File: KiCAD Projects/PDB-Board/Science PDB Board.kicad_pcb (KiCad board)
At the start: 2 copper layers, 85.1 x 63.5 mm, 8 parts, among them P1 MOTOR_PWR_OUT, P2 MAIN_PWR_IN, P3 5V_OUT, P4 PWR_REG

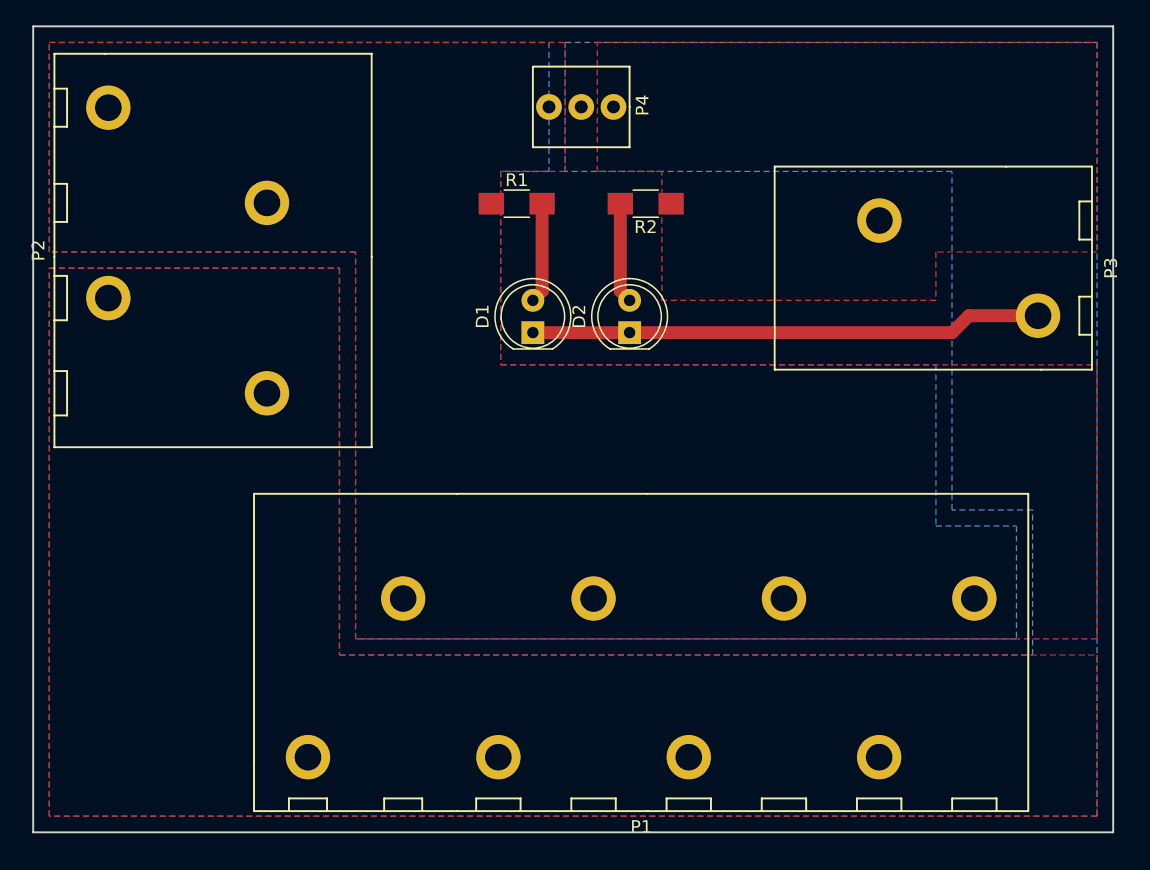
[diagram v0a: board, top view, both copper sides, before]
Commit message: Finished? PDB v2
Committing this that weren't?
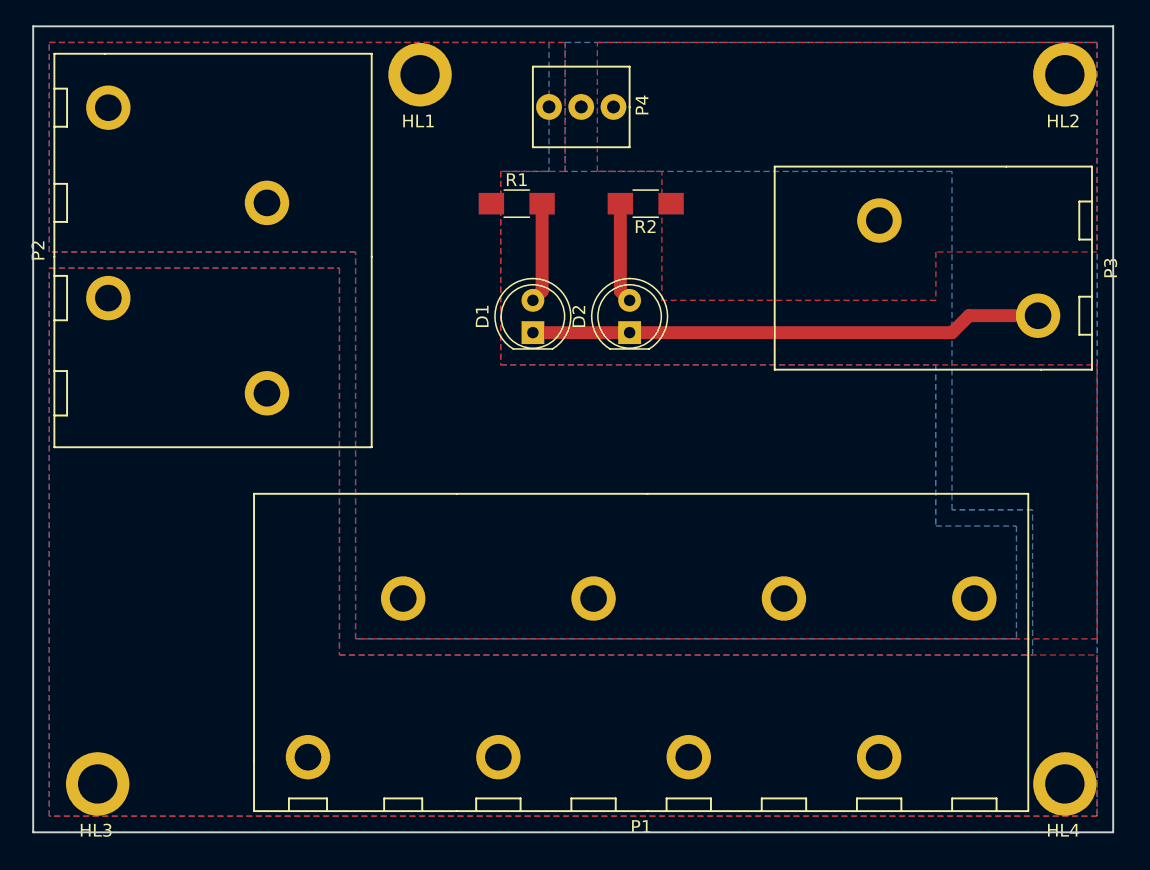
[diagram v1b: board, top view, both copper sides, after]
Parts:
- added HL1: HOLE, hole:HOLE_M3, F.Cu at (144.8, 80.0)
- added HL2: HOLE, hole:HOLE_M3, F.Cu at (195.6, 80.0)
- added HL3: HOLE, hole:HOLE_M3, F.Cu at (119.4, 135.9)
- added HL4: HOLE, hole:HOLE_M3, F.Cu at (195.6, 135.9)
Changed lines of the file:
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@@
 (kicad_pcb (version 4) (host pcbnew 4.0.3-stable)
   (general
-    (links 20)
-    (no_connects 0)
+    (links 24)
+    (no_connects 1)
     (area 114.224999 76.124999 199.465001 139.775001)
     (thickness 1.6)
@@
     (tracks 8)
     (zones 0)
-    (modules 8)
+    (modules 12)
     (nets 6)
   )
@@
   )
   (setup
-    (last_trace_width 1.016)
+    (last_trace_width 0.25)
     (user_trace_width 1.016)
     (trace_clearance 0.2)
@@
     )
   )
+  (module hole:HOLE_M3 (layer F.Cu)
+    (at 144.78 80.01)
+    (fp_text reference HL1 (at -0.127 3.683) (layer F.SilkS)
+      (effects (font (size 1 1) (thickness 0.15)))
+    )
+    (fp_text value HOLE (at 0.127 -3.683) (layer F.Fab)
+      (effects (font (size 1 1) (thickness 0.15)))
+    )
+    (pad 1 thru_hole circle (at 0 0) (size 5 5) (drill 3.1) (layers *.Cu *.Mask)
+      (net 5 GND))
+  )
+  (module hole:HOLE_M3 (layer F.Cu)
+    (at 195.58 80.01)
+    (fp_text reference HL2 (at -0.127 3.683) (layer F.SilkS)
+      (effects (font (size 1 1) (thickness 0.15)))
+    )
+    (fp_text value HOLE (at 0.127 -3.683) (layer F.Fab)
+      (effects (font (size 1 1) (thickness 0.15)))
+    )
+    (pad 1 thru_hole circle (at 0 0) (size 5 5) (drill 3.1) (layers *.Cu *.Mask)
+      (net 5 GND))
+  )
+  (module hole:HOLE_M3 (layer F.Cu)
+    (at 119.38 135.89)
+    (fp_text reference HL3 (at -0.127 3.683) (layer F.SilkS)
+      (effects (font (size 1 1) (thickness 0.15)))
+    )
+    (fp_text value HOLE (at 0.127 -3.683) (layer F.Fab)
+      (effects (font (size 1 1) (thickness 0.15)))
+    )
+    (pad 1 thru_hole circle (at 0 0) (size 5 5) (drill 3.1) (layers *.Cu *.Mask)
+      (net 5 GND))
+  )
+  (module hole:HOLE_M3 (layer F.Cu)
+    (at 195.58 135.89)
+    (fp_text reference HL4 (at -0.127 3.683) (layer F.SilkS)
+      (effects (font (size 1 1) (thickness 0.15)))
+    )
+    (fp_text value HOLE (at 0.127 -3.683) (layer F.Fab)
+      (effects (font (size 1 1) (thickness 0.15)))
+    )
+    (pad 1 thru_hole circle (at 0 0) (size 5 5) (drill 3.1) (layers *.Cu *.Mask)
+      (net 5 GND))
+  )
   (gr_line (start 114.3 139.7) (end 114.3 76.2) (angle 90) (layer Edge.Cuts) (width 0.15))
   (gr_line (start 199.39 139.7) (end 114.3 139.7) (angle 90) (layer Edge.Cuts) (width 0.15))
@@
   (segment (start 160.56 90.17) (end 160.56 97.06) (width 1.016) (layer F.Cu) (net 4))
   (segment (start 160.56 97.06) (end 161.29 97.79) (width 1.016) (layer F.Cu) (net 4))
-  (segment (start 153.67 100.33) (end 161.29 100.33) (width 1.016) (layer F.Cu) (net 5) (status C00000))
-  (segment (start 161.29 100.33) (end 186.69 100.33) (width 1.016) (layer F.Cu) (net 5) (status 400000))
+  (segment (start 153.67 100.33) (end 161.29 100.33) (width 1.016) (layer F.Cu) (net 5))
+  (segment (start 161.29 100.33) (end 186.69 100.33) (width 1.016) (layer F.Cu) (net 5))
   (segment (start 186.69 100.33) (end 188.02 99) (width 1.016) (layer F.Cu) (net 5))
-  (segment (start 188.02 99) (end 193.47 99) (width 1.016) (layer F.Cu) (net 5) (status 800000))
+  (segment (start 188.02 99) (end 193.47 99) (width 1.016) (layer F.Cu) (net 5))
   (zone (net 3) (net_name +5V) (layer F.Cu) (hatch edge 0.508)
     (connect_pads (clearance 0.508))

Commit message: Revert "Finished? PDB v2"
This reverts commit a04adeda8b22dfbdd33fba7944ab085dcccc9394.
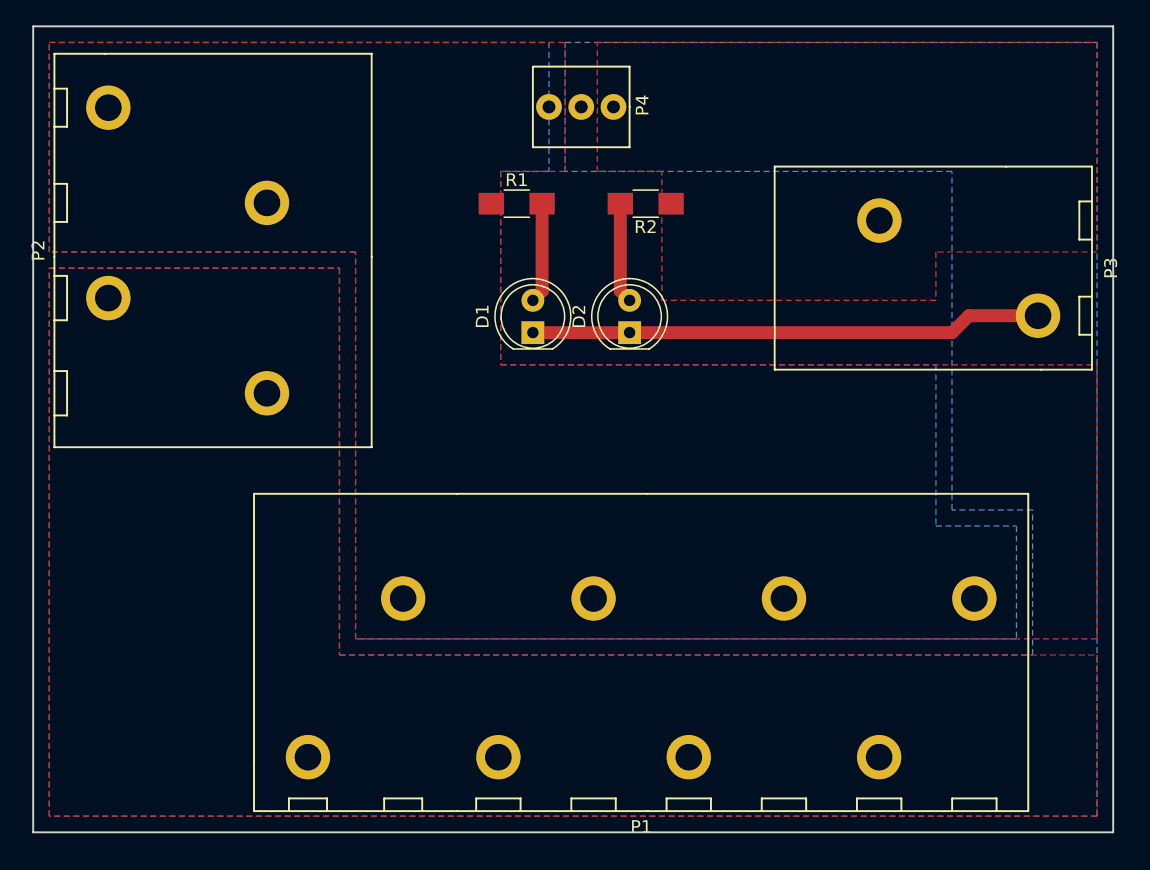
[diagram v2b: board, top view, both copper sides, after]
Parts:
- removed HL1, HL2, HL3, HL4: HOLE, hole:HOLE_M3
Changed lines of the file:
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@@
 (kicad_pcb (version 4) (host pcbnew 4.0.3-stable)
   (general
-    (links 24)
-    (no_connects 1)
+    (links 20)
+    (no_connects 0)
     (area 114.224999 76.124999 199.465001 139.775001)
     (thickness 1.6)
@@
     (tracks 8)
     (zones 0)
-    (modules 12)
+    (modules 8)
     (nets 6)
   )
@@
   )
   (setup
-    (last_trace_width 0.25)
+    (last_trace_width 1.016)
     (user_trace_width 1.016)
     (trace_clearance 0.2)
@@
     )
   )
-  (module hole:HOLE_M3 (layer F.Cu)
-    (at 144.78 80.01)
-    (fp_text reference HL1 (at -0.127 3.683) (layer F.SilkS)
-      (effects (font (size 1 1) (thickness 0.15)))
-    )
-    (fp_text value HOLE (at 0.127 -3.683) (layer F.Fab)
-      (effects (font (size 1 1) (thickness 0.15)))
-    )
-    (pad 1 thru_hole circle (at 0 0) (size 5 5) (drill 3.1) (layers *.Cu *.Mask)
-      (net 5 GND))
-  )
-  (module hole:HOLE_M3 (layer F.Cu)
-    (at 195.58 80.01)
-    (fp_text reference HL2 (at -0.127 3.683) (layer F.SilkS)
-      (effects (font (size 1 1) (thickness 0.15)))
-    )
-    (fp_text value HOLE (at 0.127 -3.683) (layer F.Fab)
-      (effects (font (size 1 1) (thickness 0.15)))
-    )
-    (pad 1 thru_hole circle (at 0 0) (size 5 5) (drill 3.1) (layers *.Cu *.Mask)
-      (net 5 GND))
-  )
-  (module hole:HOLE_M3 (layer F.Cu)
-    (at 119.38 135.89)
-    (fp_text reference HL3 (at -0.127 3.683) (layer F.SilkS)
-      (effects (font (size 1 1) (thickness 0.15)))
-    )
-    (fp_text value HOLE (at 0.127 -3.683) (layer F.Fab)
-      (effects (font (size 1 1) (thickness 0.15)))
-    )
-    (pad 1 thru_hole circle (at 0 0) (size 5 5) (drill 3.1) (layers *.Cu *.Mask)
-      (net 5 GND))
-  )
-  (module hole:HOLE_M3 (layer F.Cu)
-    (at 195.58 135.89)
-    (fp_text reference HL4 (at -0.127 3.683) (layer F.SilkS)
-      (effects (font (size 1 1) (thickness 0.15)))
-    )
-    (fp_text value HOLE (at 0.127 -3.683) (layer F.Fab)
-      (effects (font (size 1 1) (thickness 0.15)))
-    )
-    (pad 1 thru_hole circle (at 0 0) (size 5 5) (drill 3.1) (layers *.Cu *.Mask)
-      (net 5 GND))
-  )
   (gr_line (start 114.3 139.7) (end 114.3 76.2) (angle 90) (layer Edge.Cuts) (width 0.15))
   (gr_line (start 199.39 139.7) (end 114.3 139.7) (angle 90) (layer Edge.Cuts) (width 0.15))
@@
   (segment (start 160.56 90.17) (end 160.56 97.06) (width 1.016) (layer F.Cu) (net 4))
   (segment (start 160.56 97.06) (end 161.29 97.79) (width 1.016) (layer F.Cu) (net 4))
-  (segment (start 153.67 100.33) (end 161.29 100.33) (width 1.016) (layer F.Cu) (net 5))
-  (segment (start 161.29 100.33) (end 186.69 100.33) (width 1.016) (layer F.Cu) (net 5))
+  (segment (start 153.67 100.33) (end 161.29 100.33) (width 1.016) (layer F.Cu) (net 5) (status C00000))
+  (segment (start 161.29 100.33) (end 186.69 100.33) (width 1.016) (layer F.Cu) (net 5) (status 400000))
   (segment (start 186.69 100.33) (end 188.02 99) (width 1.016) (layer F.Cu) (net 5))
-  (segment (start 188.02 99) (end 193.47 99) (width 1.016) (layer F.Cu) (net 5))
+  (segment (start 188.02 99) (end 193.47 99) (width 1.016) (layer F.Cu) (net 5) (status 800000))
   (zone (net 3) (net_name +5V) (layer F.Cu) (hatch edge 0.508)
     (connect_pads (clearance 0.508))
